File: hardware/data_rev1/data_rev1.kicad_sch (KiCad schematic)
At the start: 2 parts, among them J1 BOARD, U1 Pico

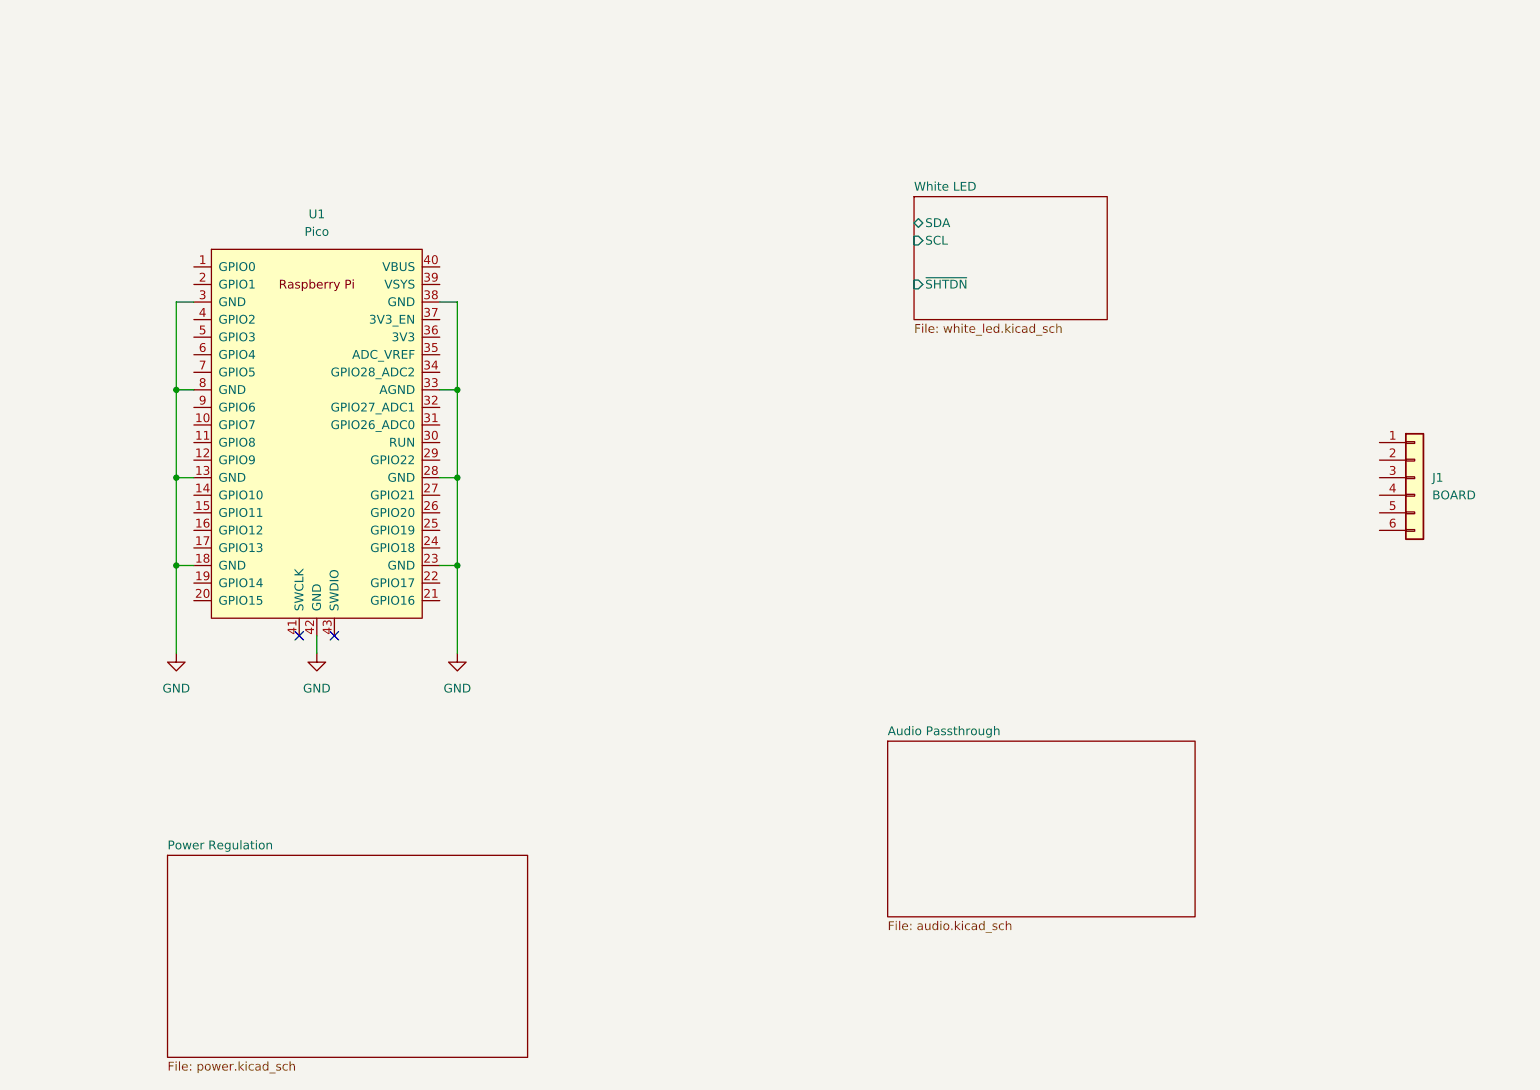
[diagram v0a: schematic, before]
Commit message: Initial layout and circuit
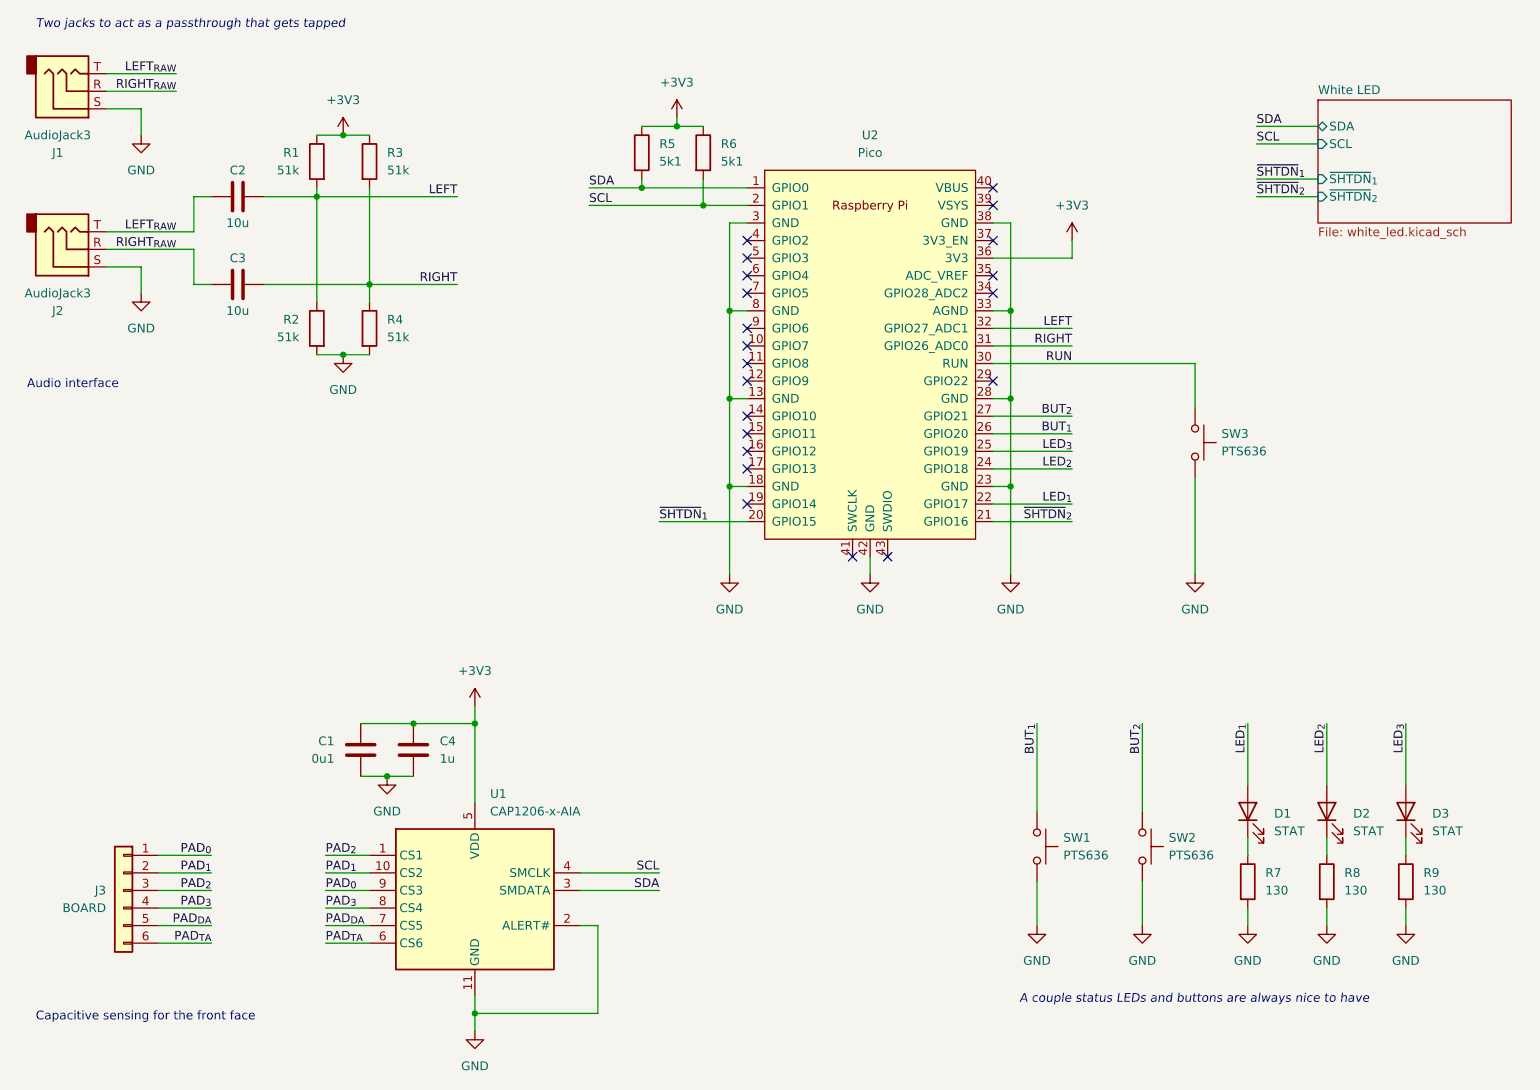
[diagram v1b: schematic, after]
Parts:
- added C1: 0u1, Capacitor_SMD:C_0603_1608Metric, symbol Device:C
- added C2, C3: 10u, Resistor_SMD:R_0805_2012Metric, symbol Device:C
- added C4: 1u, Capacitor_SMD:C_0603_1608Metric, symbol Device:C
- added D1, D2, D3: STAT, LED_SMD:LED_0805_2012Metric, symbol Device:LED
- added J1, J2: AudioJack3, Connector_Audio:Jack_3.5mm_CUI_SJ-3523-SMT_Horizontal, symbol Connector_Audio:AudioJack3
- added R1, R2, R3, R4: 51k, Resistor_SMD:R_0603_1608Metric, symbol Device:R
- added R5, R6: 5k1, Resistor_SMD:R_0603_1608Metric, symbol Device:R
- added R7, R8, R9: 130, Resistor_SMD:R_0603_1608Metric, symbol Device:R
- added SW1, SW2, SW3: PTS636, Button_Switch_SMD:SW_SPST_CK_RS282G05A3, symbol Switch:SW_Push
- added U1: CAP1206-x-AIA, Package_DFN_QFN:DFN-10-1EP_3x3mm_P0.5mm_EP1.55x2.48mm, symbol Sensor_Touch:CAP1206-x-AIA
- renumbered J1 to J3, U1 to U2
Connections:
- net GND: now also C1.2, C4.1, J1.S, J2.S, R2.2, R4.2, R7.2, R8.2, R9.2, SW1.2, SW2.2, SW3.2, U1.11 (GND), U1.2 (ALERT#)
- net SDA: now reaches U2.1 (GPIO0)
- net SDA: now also R5.2, U1.3 (SMDATA)
- net SCL: now reaches U2.2 (GPIO1)
- net SCL: now also R6.2, U1.4 (SMCLK)
- net ~{SHTDN}_{1}: now reaches U2.20 (GPIO15)
- net ~{SHTDN}_{2}: now reaches U2.21 (GPIO16)
- net LED_{1}: now reaches U2.22 (GPIO17)
- net LED_{1}: now also D1.2 (A)
- net LED_{2}: now reaches U2.24 (GPIO18)
- net LED_{2}: now also D2.2 (A)
- net LED_{3}: now reaches U2.25 (GPIO19)
- net LED_{3}: now also D3.2 (A)
- net BUT_{1}: now reaches U2.26 (GPIO20)
- net BUT_{1}: now also SW1.1
- net BUT_{2}: now reaches U2.27 (GPIO21)
- net BUT_{2}: now also SW2.1
- net RUN: now reaches U2.30 (RUN)
- net RUN: now also SW3.1
- net RIGHT: now reaches U2.31 (GPIO26_ADC0)
- net RIGHT: now also C3.1, R3.2, R4.1
- net LEFT: now reaches U2.32 (GPIO27_ADC1)
- net LEFT: now also C2.1, R1.2, R2.1
- net +3V3: now reaches U2.36 (3V3)
- net +3V3: now also C1.1, C4.2, R1.1, R3.1, R5.1, R6.1, U1.5 (VDD)
- net PAD_{0}: now reaches J3.1 (Pin_1)
- net PAD_{0}: now also U1.9 (CS3)
- net PAD_{1}: now reaches J3.2 (Pin_2)
- net PAD_{1}: now also U1.10 (CS2)
- net PAD_{2}: now reaches J3.3 (Pin_3)
- net PAD_{2}: now also U1.1 (CS1)
- net PAD_{3}: now reaches J3.4 (Pin_4)
- net PAD_{3}: now also U1.8 (CS4)
- net PAD_{DA}: now reaches J3.5 (Pin_5)
- net PAD_{DA}: now also U1.7 (CS5)
- net PAD_{TA}: now reaches J3.6 (Pin_6)
- net PAD_{TA}: now also U1.6 (CS6)
- new net: D3.1 (K), R9.1
- new net: D2.1 (K), R8.1
- new net: D1.1 (K), R7.1
- new net LEFT_{RAW}: C2.2, J1.T, J2.T
- new net RIGHT_{RAW}: C3.2, J1.R, J2.R
- no-connect marks 2 -> 21
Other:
- removed sheet Audio Passthrough
- removed sheet Power Regulation
- sheet White LED ports: added ~{SHTDN}_{1}, ~{SHTDN}_{2}; removed ~{SHTDN}
- note added: "A couple status LEDs and buttons are always nice to have"
- note added: "Audio interface"
- note added: "Capacitive sensing for the front face"
- note added: "Two jacks to act as a passthrough that gets tapped"
- moved on the sheet: J3, U2
